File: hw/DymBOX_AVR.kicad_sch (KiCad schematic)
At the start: 45 parts, among them J1 Conn_01x01_Pin, J2 Conn_01x01_Pin, J3 Conn_01x01_Pin, J4 DS18B20, J5 Conn_02x05_Odd_Even, J6 Conn_01x01_Pin, K1 RT314A24, Q1 BC327, Q2 BC327, Q3 BS170, Q4 BS170, Q5 BC327, SW1 RotaryEncoder_Switch, U1 ATmega8A-P, U2 CA56-12EWA, U3 L7805, Y1 16MHz

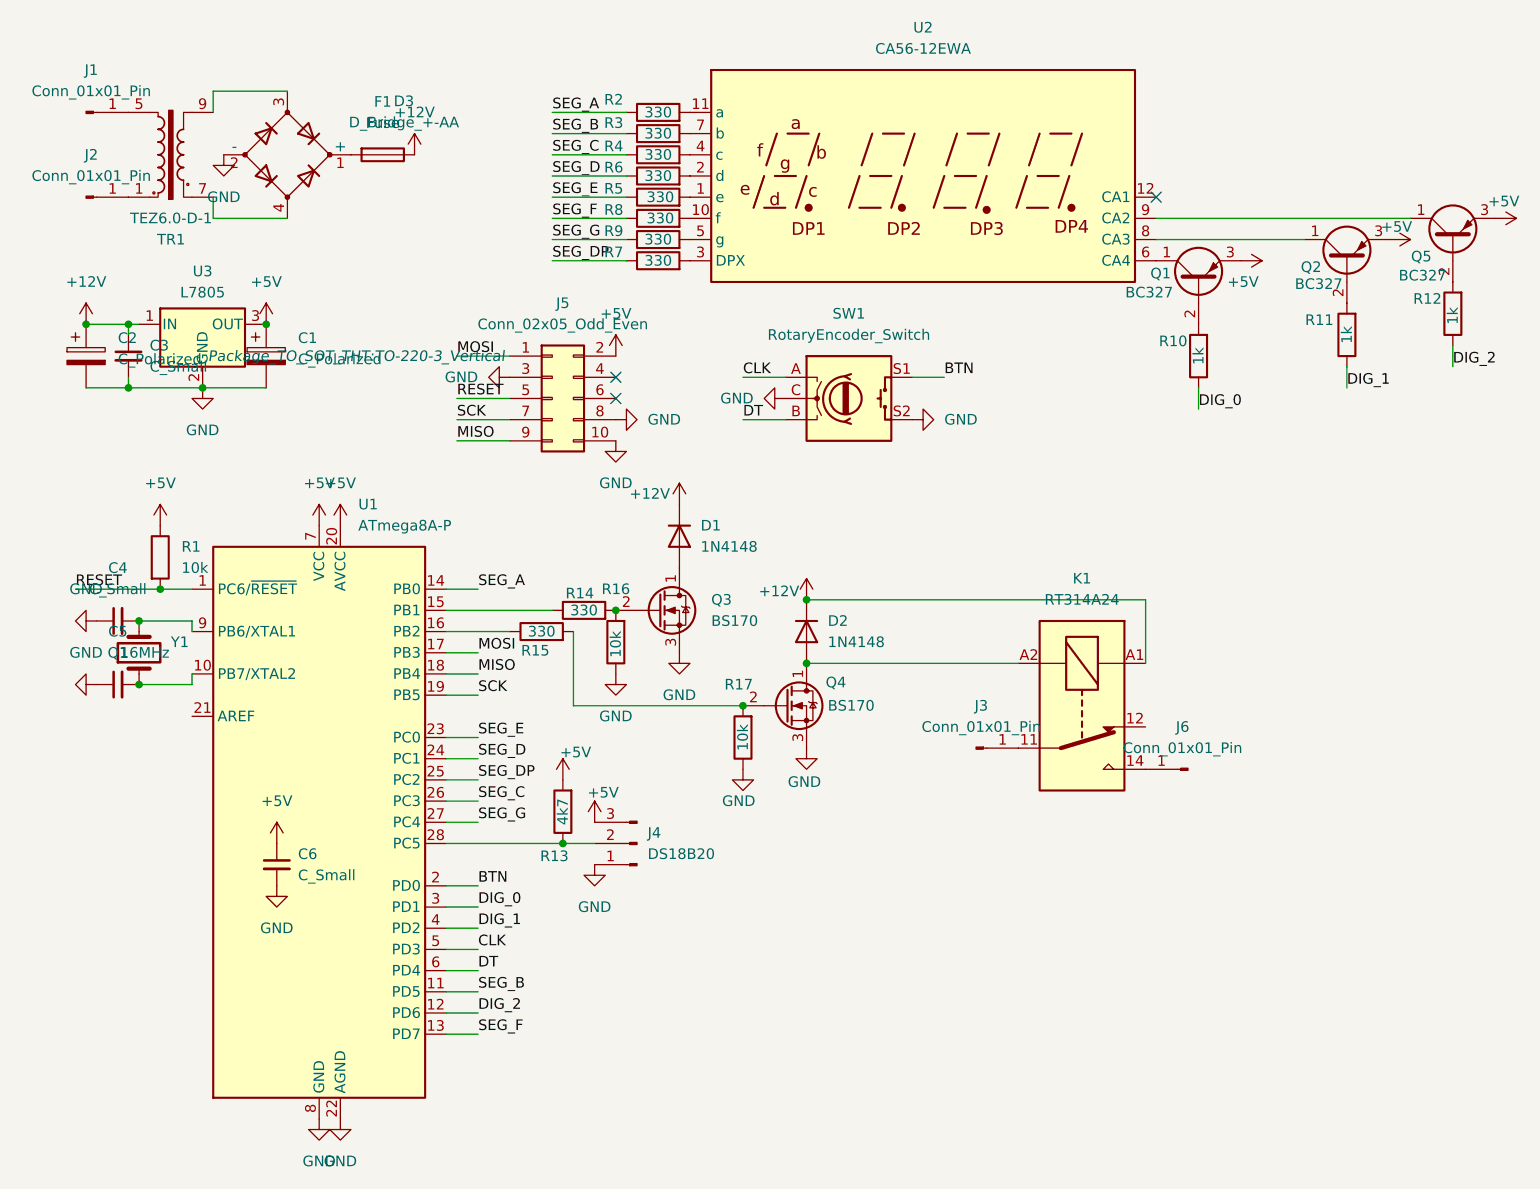
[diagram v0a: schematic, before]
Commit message: uprava a více
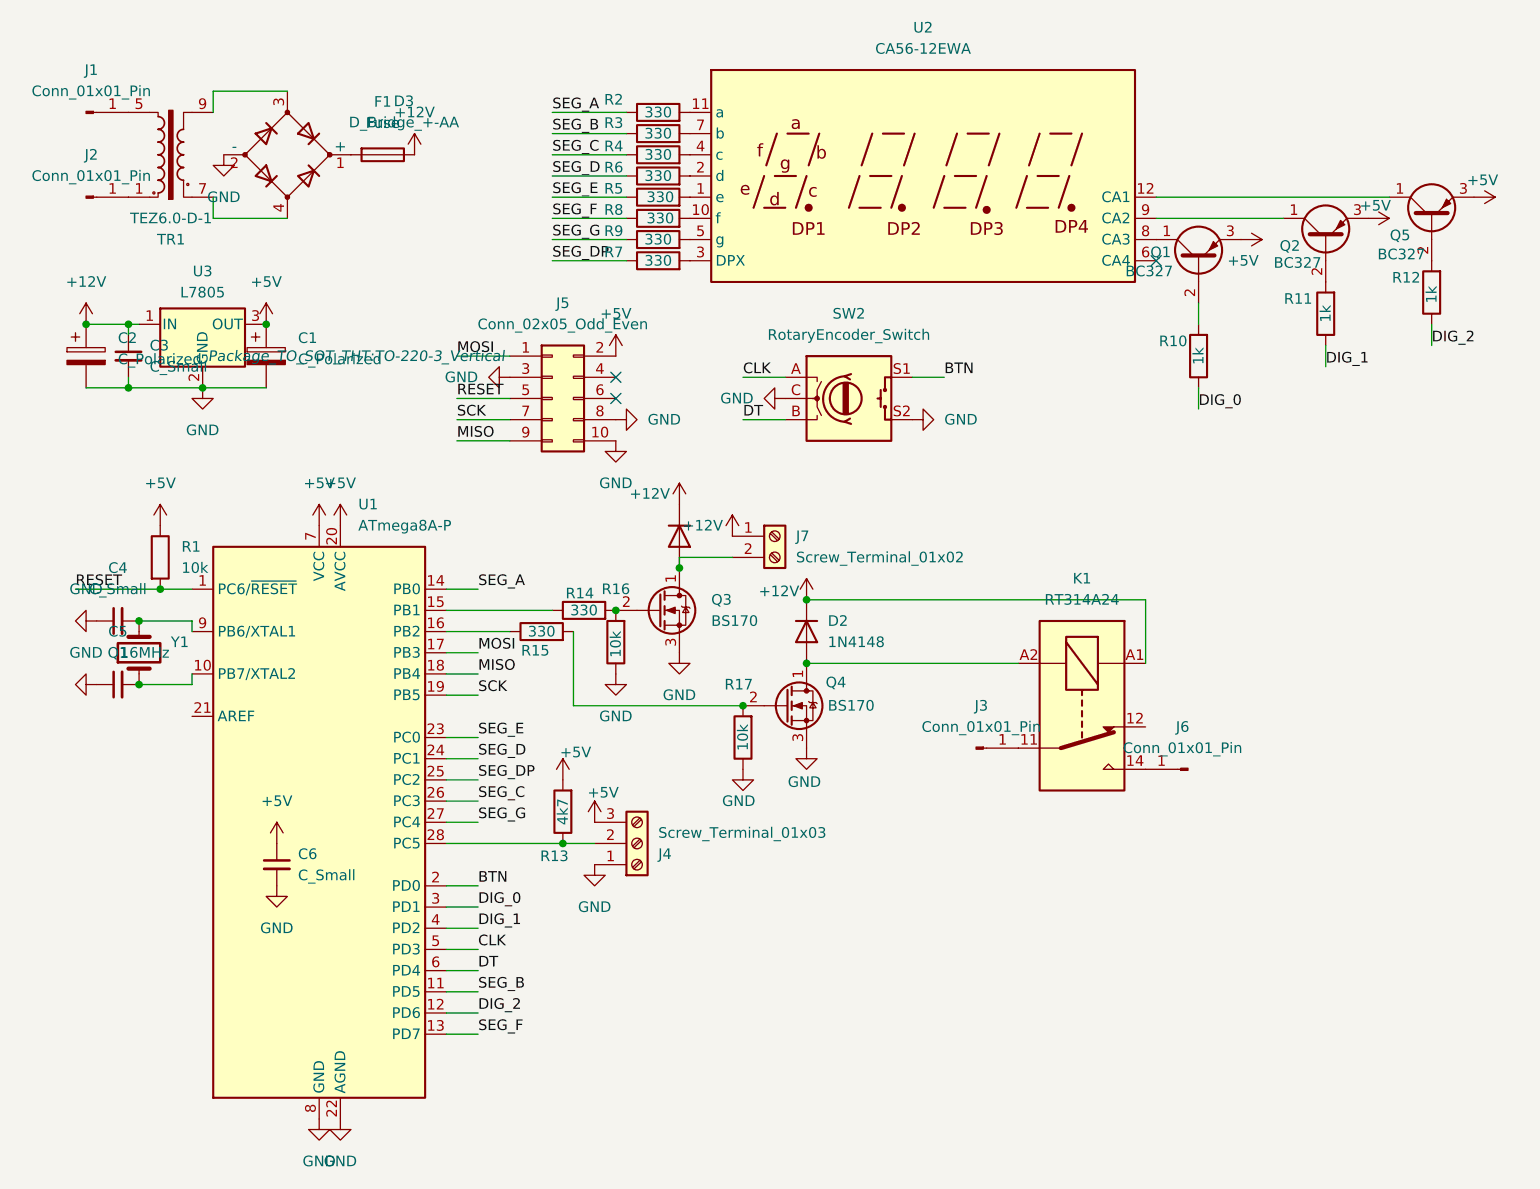
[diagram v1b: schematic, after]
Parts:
- removed J4: DS18B20, Connector_Wire:SolderWire-0.127sqmm_1x03_P3.7mm_D0.48mm_OD1mm, symbol Connector:Conn_01x03_Pin
- removed SW1: RotaryEncoder_Switch, 2pkstartup:RotaryEncoder_Alps_EC12E-Switch_Vertical_H20mm_CircularMountingHoles, symbol Device:RotaryEncoder_Switch
- added J4: Screw_Terminal_01x03, TerminalBlock_Phoenix:TerminalBlock_Phoenix_PT-1,5-3-3.5-H_1x03_P3.50mm_Horizontal, symbol Connector:Screw_Terminal_01x03
- added J7: Screw_Terminal_01x02, TerminalBlock_Phoenix:TerminalBlock_Phoenix_PT-1,5-2-3.5-H_1x02_P3.50mm_Horizontal, symbol Connector:Screw_Terminal_01x02
- added SW2: RotaryEncoder_Switch, 2pkstartup:RotaryEncoder_Alps_EC12E-Switch_Vertical_H20mm_CircularMountingHoles, symbol 2pkstartup:RotaryEncoder_Switch
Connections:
- net +12V: now also J7.1 (Pin_1)
- net +5V: now also J4.3 (Pin_3)
- net BTN: now also SW2.S1
- net CLK: now also SW2.A
- net DT: now also SW2.B
- net GND: now also J4.1 (Pin_1), SW2.C, SW2.S2
- net at D1.2 (A), Q3.1 (D): now also J7.2 (Pin_2)
- net at R13.1, U1.28 (PC5): now also J4.2 (Pin_2)
- net at Q1.1 (C): now also U2.8 (CA3); no longer U2.6 (CA4)
- net at Q2.1 (C): now also U2.9 (CA2); no longer U2.8 (CA3)
- net at Q5.1 (C): now also U2.12 (CA1); no longer U2.9 (CA2)
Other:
- moved on the sheet: Q1, Q2, Q5, R11, R12

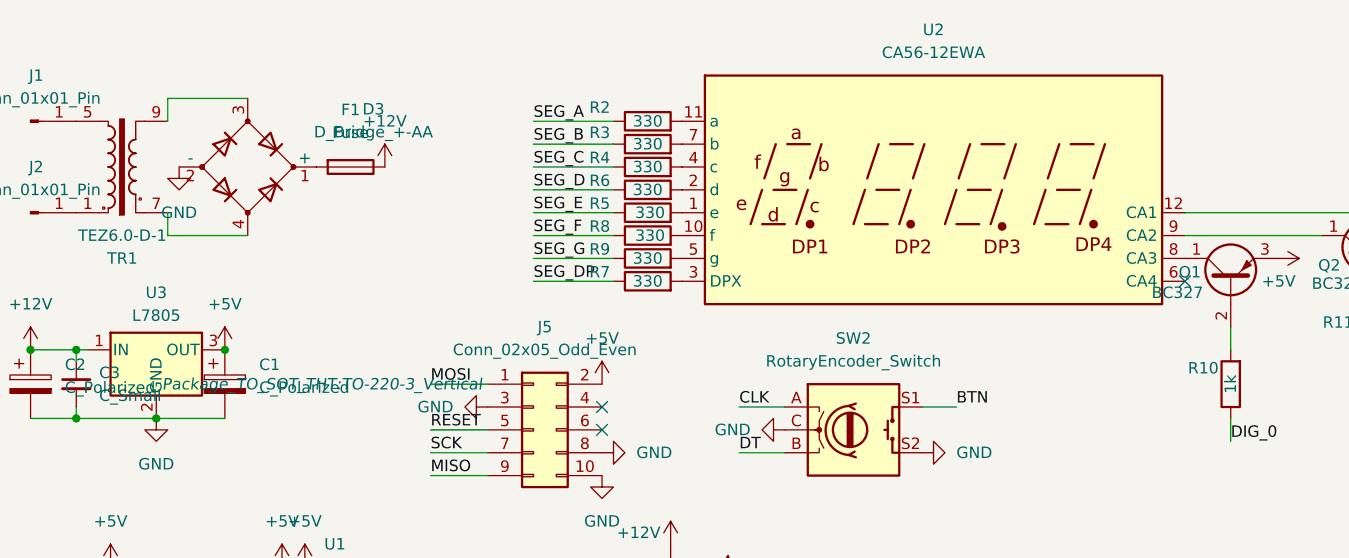
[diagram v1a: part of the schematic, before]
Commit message: AP63005
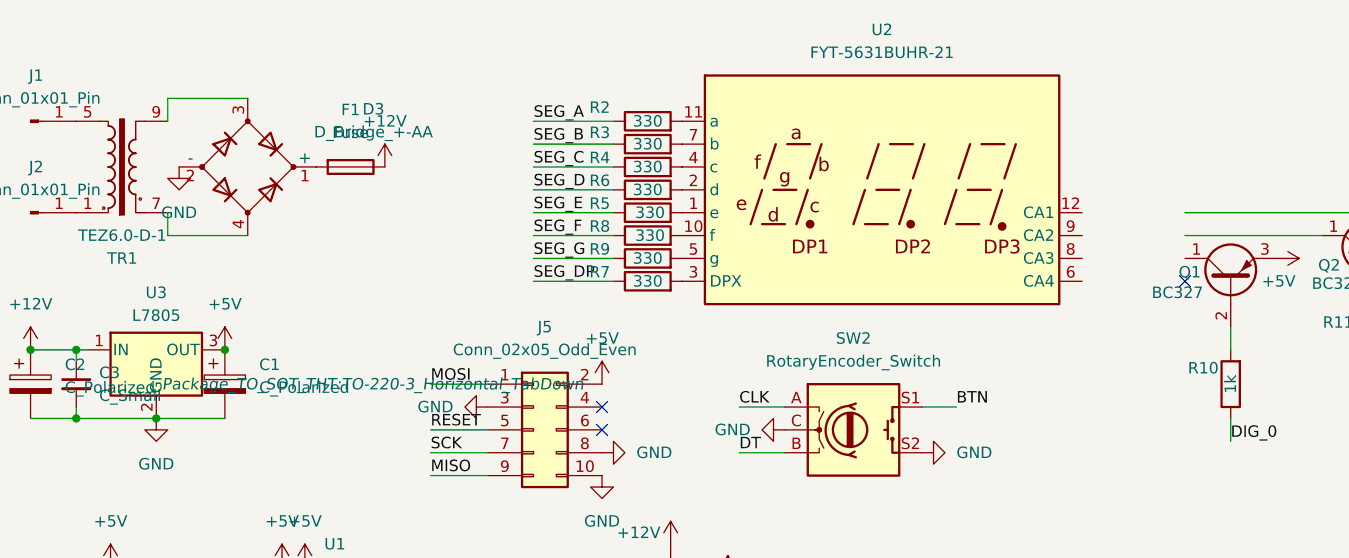
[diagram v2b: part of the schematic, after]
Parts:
- removed U2: CA56-12EWA, Display_7Segment:CA56-12EWA, symbol Display_Character:CA56-12EWA
- added U2: FYT-5631BUHR-21, 2pkstartup:FYT-5631BUHR-21, symbol 2pkstartup:FYT-5631BUHR-21
- C1, C2: footprint Capacitor_THT:CP_Radial_D13.0mm_P5.00mm -> Capacitor_THT:CP_Radial_D16.0mm_P7.50mm
- U3: footprint Package_TO_SOT_THT:TO-220-3_Vertical -> Package_TO_SOT_THT:TO-220-3_Horizontal_TabDown
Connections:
- net at R7.2: now also U2.3 (DPX)
- net at R6.2: now also U2.2 (d)
- net at R8.2: now also U2.10 (f)
- net at R9.2: now also U2.5 (g)
- net at R2.2: now also U2.11 (a)
- net at R3.2: now also U2.7 (b)
- net at R5.2: now also U2.1 (e)
- net at R4.2: now also U2.4 (c)
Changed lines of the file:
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@@
 			)
 		)
-		(property "Footprint" "Package_TO_SOT_THT:TO-220-3_Vertical"
+		(property "Footprint" "Package_TO_SOT_THT:TO-220-3_Horizontal_TabDown"
 			(at 53.975 64.77 0)
 			(show_name no)
@@
 			)
 		)
-		(property "Footprint" "Capacitor_THT:CP_Radial_D13.0mm_P5.00mm"
+		(property "Footprint" "Capacitor_THT:CP_Radial_D16.0mm_P7.50mm"
 			(at 40.3352 68.58 0)
 			(hide yes)
@@
 			)
 		)
-		(property "Footprint" "Capacitor_THT:CP_Radial_D13.0mm_P5.00mm"
+		(property "Footprint" "Capacitor_THT:CP_Radial_D16.0mm_P7.50mm"
 			(at 61.9252 68.58 0)
 			(hide yes)
@@
 	)
 	(symbol
-		(lib_id "Display_Character:CA56-12EWA")
-		(at 139.7 43.18 0)
-		(unit 1)
-		(body_style 1)
-		(exclude_from_sim no)
-		(in_bom yes)
-		(on_board yes)
-		(in_pos_files yes)
-		(dnp no)
-		(fields_autoplaced yes)
-		(property "Reference" "U2"
-			(at 139.7 25.4 0)
-			(show_name no)
-			(do_not_autoplace no)
-			(effects
-				(font
-					(size 1.27 1.27)
-				)
-			)
-		)
-		(property "Value" "CA56-12EWA"
-			(at 139.7 27.94 0)
-			(show_name no)
-			(do_not_autoplace no)
-			(effects
-				(font
-					(size 1.27 1.27)
-				)
-			)
-		)
-		(property "Footprint" "Display_7Segment:CA56-12EWA"
-			(at 139.7 58.42 0)
-			(hide yes)
-			(show_name no)
-			(do_not_autoplace no)
-			(effects
-				(font
-					(size 1.27 1.27)
-				)
-			)
-		)
-		(property "Datasheet" "http://www.kingbrightusa.com/images/catalog/SPEC/CA56-12EWA.pdf"
-			(at 128.778 42.418 0)
-			(hide yes)
-			(show_name no)
-			(do_not_autoplace no)
-			(effects
-				(font
-					(size 1.27 1.27)
-				)
-			)
-		)
-		(property "Description" "4 digit 7 segment high efficiency red LED, common anode"
-			(at 139.7 43.18 0)
-			(hide yes)
-			(show_name no)
-			(do_not_autoplace no)
-			(effects
-				(font
-					(size 1.27 1.27)
-				)
-			)
-		)
-		(pin "10"
-		)
-		(pin "3"
-		)
-		(pin "11"
-		)
-		(pin "9"
-		)
-		(pin "8"
-		)
-		(pin "12"
-		)
-		(pin "6"
-		)
-		(pin "4"
-		)
-		(pin "7"
-		)
-		(pin "5"
-		)
-		(pin "1"
-		)
-		(pin "2"
-		)
-		(instances
-			(project "DymBOX_AVR"
-				(path "/586f9677-488d-4753-8c82-bcf4ec642766"
-					(reference "U2")
-					(unit 1)
-				)
-			)
-		)
-	)
-	(symbol
 		(lib_id "Device:R")
 		(at 118.11 110.49 180)
@@
 					(unit 1)
 				)
+			)
+		)
+	)
+	(symbol
+		(lib_id "2pkstartup:FYT-5631BUHR-21")
+		(at 139.7 43.18 0)
+		(unit 1)
+		(body_style 1)
+		(exclude_from_sim no)
+		(in_bom yes)
+		(on_board yes)
+		(in_pos_files yes)
+		(dnp no)
+		(fields_autoplaced yes)
+		(property "Reference" "U2"
+			(at 133.985 25.4 0)
+			(show_name no)
+			(do_not_autoplace no)
+			(effects
+				(font
+					(size 1.27 1.27)
+				)
+			)
+		)
+		(property "Value" "FYT-5631BUHR-21"
+			(at 133.985 27.94 0)
+			(show_name no)
+			(do_not_autoplace no)
+			(effects
+				(font
+					(size 1.27 1.27)
+				)
+			)
+		)
+		(property "Footprint" "2pkstartup:FYT-5631BUHR-21"
+			(at 139.7 58.42 0)
+			(hide yes)
+			(show_name no)
+			(do_not_autoplace no)
+			(effects
+				(font
+					(size 1.27 1.27)
+				)
+			)
+		)
+		(property "Datasheet" "https://cetest02.cn-bj.ufileos.com/100001_2003185297/20%20FYT-5631A-BX-XX.pdf"
+			(at 128.778 42.418 0)
+			(hide yes)
+			(show_name no)
+			(do_not_autoplace no)
+			(effects
+				(font
+					(size 1.27 1.27)
+				)
+			)
+		)
+		(property "Description" "3 digit 7 segment high efficiency red LED, common anode"
+			(at 139.7 43.18 0)
+			(hide yes)
+			(show_name no)
+			(do_not_autoplace no)
+			(effects
+				(font
+					(size 1.27 1.27)
+				)
+			)
+		)
+		(pin "3"
+		)
+		(pin "1"
+		)
+		(pin "4"
+		)
+		(pin "2"
+		)
+		(pin "9"
+		)
+		(pin "5"
+		)
+		(pin "8"
+		)
+		(pin "7"
+		)
+		(pin "10"
+		)
+		(pin "6"
+		)
+		(pin "11"
+		)
+		(pin "12"
+		)
+		(instances
+			(project "DymBOX_AVR"
+				(path "/586f9677-488d-4753-8c82-bcf4ec642766"
+					(reference "U2")
+					(unit 1)
+				)
